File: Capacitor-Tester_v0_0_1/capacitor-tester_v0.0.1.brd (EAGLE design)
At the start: 67 x 45 mm, 34 parts, among them IC1 AD8531ARZ, IC2 MC34063EBD-TR, IC3 DAC6571IDBVT, IC5 AD8397ARDZ, J1 USB4125-GF-A-0190_REVA2, J2 DS1044-140G, J4 250-103, U1 AD5933, Y1 LFSPXO018034

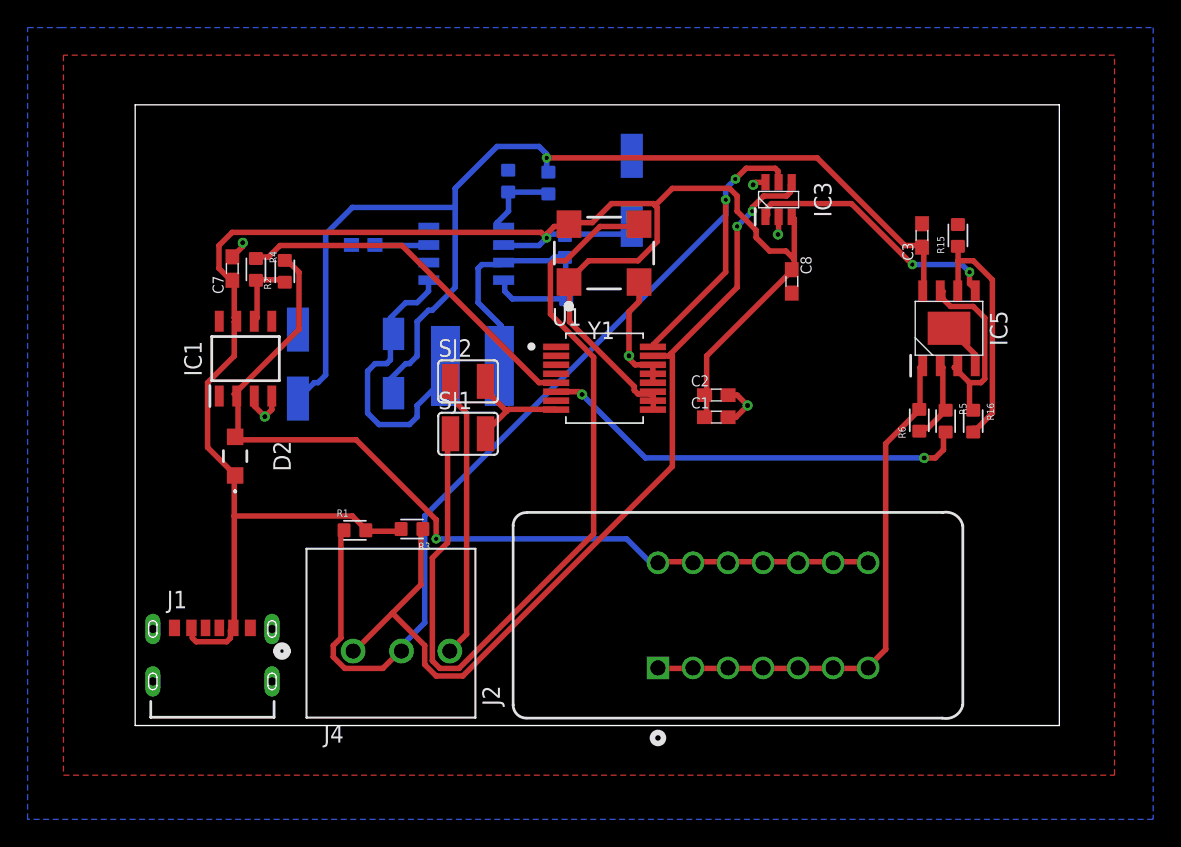
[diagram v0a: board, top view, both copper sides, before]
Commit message: v0.0.1 - CMD renumber + tnames + bnames
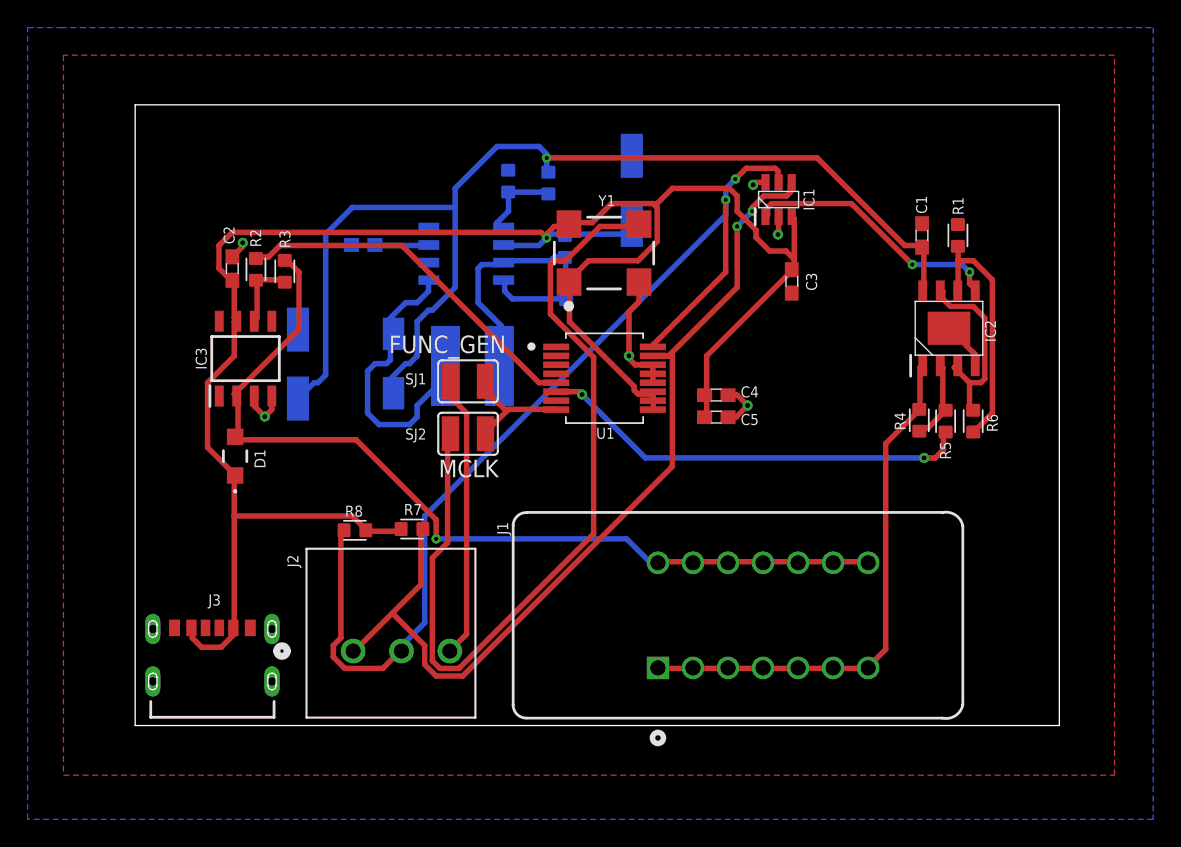
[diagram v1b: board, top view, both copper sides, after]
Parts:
- removed IC5: AD8397ARDZ, AD8397ARDZ:SOIC127P600X175-9N
- removed J4: 250-103, custom_library:CONN3_250-103_WAG
- removed R15, R16: 10k-1%, custom_library:R0603
- added IC4: MC34063EBD-TR, MC34063EBD-TR:SOIC127P600X175-8N
- added J3: USB4125-GF-A-0190_REVA2, USB-C-6Pin:GCT_USB4125-GF-A-0190_REVA2
- added R7, R8: DNP-4k7-1%, custom_library:R0603
- C2: value 10u -> 100n
- C3: value 100n -> 10u
- C4: value 270u / 16V -> 10u; device EEEFKC271XSP:EEE0JA331XP -> custom_library:C0603
- C5: value 270u / 16V -> 100n; device EEEFKC271XSP:EEE0JA331XP -> custom_library:C0603
- C6: value 560p -> 270u / 16V; device custom_library:C0603 -> EEEFKC271XSP:EEE0JA331XP
- C7: value 100n -> 560p
- C8: value 10u -> 270u / 16V; device custom_library:C0603 -> EEEFKC271XSP:EEE0JA331XP
- D1: value SS14 -> PMEG6020ER,115; device SS14:DIOM5227X270N -> PMEG6020ER_115:PMEG6020ER115
- D2: value PMEG6020ER,115 -> SS14; device PMEG6020ER_115:PMEG6020ER115 -> SS14:DIOM5227X270N
- IC1: value AD8531ARZ -> DAC6571IDBVT; device AD8531ARZ:SOIC127P600X175-8N -> DAC6571IDBVT:SOT95P280X145-6N
- IC2: value MC34063EBD-TR -> AD8397ARDZ; device MC34063EBD-TR:SOIC127P600X175-8N -> AD8397ARDZ:SOIC127P600X175-9N
- IC3: value DAC6571IDBVT -> AD8531ARZ; device DAC6571IDBVT:SOT95P280X145-6N -> AD8531ARZ:SOIC127P600X175-8N
- J1: value USB4125-GF-A-0190_REVA2 -> DS1044-140G; device USB-C-6Pin:GCT_USB4125-GF-A-0190_REVA2 -> DS1044-140G:CONNFLY_DS1044-140G
- J2: value DS1044-140G -> 250-103; device DS1044-140G:CONNFLY_DS1044-140G -> custom_library:CONN3_250-103_WAG
- R1, R3: value DNP-4k7-1% -> 10k-1%
- R10: value 1k-1% -> R133-1%
- R11: value R133-1% -> 8k66-1%
- R12: value 180R-1% -> 1k-1%
- R2: value 10k-1% -> DNP-10k-1%
- R4: value DNP-10k-1% -> 1k-1%
- R6: value 1k-1% -> 10k-1%
- R9: value 8k66-1% -> 180R-1%
- moved R4 49.3 mm to (56.8, 22.1), turned to 90 degrees
- moved R1 48.7 mm to (59.6, 35.5), turned to 90 degrees
- moved IC1 40.3 mm to (46.6, 38.1)
- moved IC3 40.3 mm to (8.00, 26.6)
- moved J1 40.1 mm to (45.5, 7.99), turned to 90 degrees
- moved C2 36.3 mm to (7.05, 33.1), turned to 90 degrees
- moved IC2 35.4 mm to (59.0, 28.8), flipped to the top, turned to 90 degrees
- moved C4 30.4 mm to (42.1, 24.0), flipped to the top, turned to 0 degrees
- moved J2 29.8 mm to (15.8, 5.40), turned to 0 degrees
- moved R3 20.8 mm to (10.8, 32.9), turned to 90 degrees
- moved C1 19.9 mm to (57.0, 35.5), turned to 90 degrees
- moved C5 17.6 mm to (42.1, 22.4), flipped to the top, turned to 0 degrees
- moved C8 13.3 mm to (36.0, 38.8), flipped to the bottom, turned to 90 degrees
- moved D1 13.3 mm to (7.25, 19.5), flipped to the top
- moved D2 13.3 mm to (18.7, 26.2), flipped to the bottom
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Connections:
- net +12V: now also C1.1, C6.1, D2.1, IC2.8, R11.1; no longer C3.1, C4.1, D1.1, IC5.8, R9.1
- net +5V: now also C3.1, C4.1, D1.1, IC1.3, IC3.7, IC4.6, J3.A9, J3.B9, R10.1, R7.2, R8.2; no longer C1.1, C7.1, D2.1, IC1.7, IC2.6, IC3.3, J1.A9, J1.B9, R1.2, R11.1, R3.2
- net DAC_OUT: now also IC1.1, IC2.5; no longer IC3.1, IC5.5
- net FUNC_GEN: now also J2.3, SJ1.1; no longer J4.3, SJ2.1
- net GND: now also IC1.2, IC1.6, IC2.9, IC3.3, IC3.4, IC4.2, IC4.4, J3.A12, J3.B12, J3.S1, J3.S2, J3.S3, J3.S4, R1.2, R12.2; no longer IC1.3, IC1.4, IC2.2, IC3.2, IC3.6, IC5.4, IC5.9, J1.A12, J1.B12, J1.S1, J1.S2, J1.S3, J1.S4, R10.2, R15.2
- net MCLK: now also SJ2.1; no longer SJ1.1
- net N$1: now also IC3.6, R2.2, R3.1; no longer IC1.6, R2.1, R4.2
- net N$10: now also C7.1, IC4.3; no longer C6.1, IC2.3
- net N$11: now also IC4.7, R10.2, R9.2; no longer IC2.7, R11.2, R12.2
- net N$13: now also IC2.6, R1.1, R6.2; no longer IC5.6, R15.1, R16.2
- net N$4: now also IC2.2, R4.1; no longer IC5.2, R6.1
- net N$5: now also D2.2, IC4.1; no longer D1.2, IC2.1
- net N$7: now also IC4.5, R11.2, R12.1; no longer IC2.5, R10.1, R9.2
- net N$8: now also IC4.8, R9.1; no longer IC2.8, R12.1
- net SCL: now also IC1.5, J2.2, R8.1; no longer IC3.5, J4.2, R1.1
- net SDA: now also IC1.4, J2.1, R7.1; no longer IC3.4, J4.1, R3.1
- net UZA_OUT: now also IC2.1, J1.1, J1.2, J1.3, J1.4, J1.5, J1.6, J1.7, R4.2; no longer IC5.1, J2.1, J2.2, J2.3, J2.4, J2.5, J2.6, J2.7, R6.2
- net UZB_OUT: now also IC2.3, IC2.7, R6.1; no longer IC5.3, IC5.7, R16.1
- net VIN: now also R2.1; no longer R4.1
- net Z_OUT: now also D1.2, IC3.2, J1.10, J1.11, J1.12, J1.13, J1.14, J1.8, J1.9, R3.2; no longer D2.2, IC1.2, J2.10, J2.11, J2.12, J2.13, J2.14, J2.8, J2.9, R2.2
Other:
- board text added: "FUNC_GEN"
- board text added: "MCLK"

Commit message: v0.0.1 - Revert to commit b06d3d6
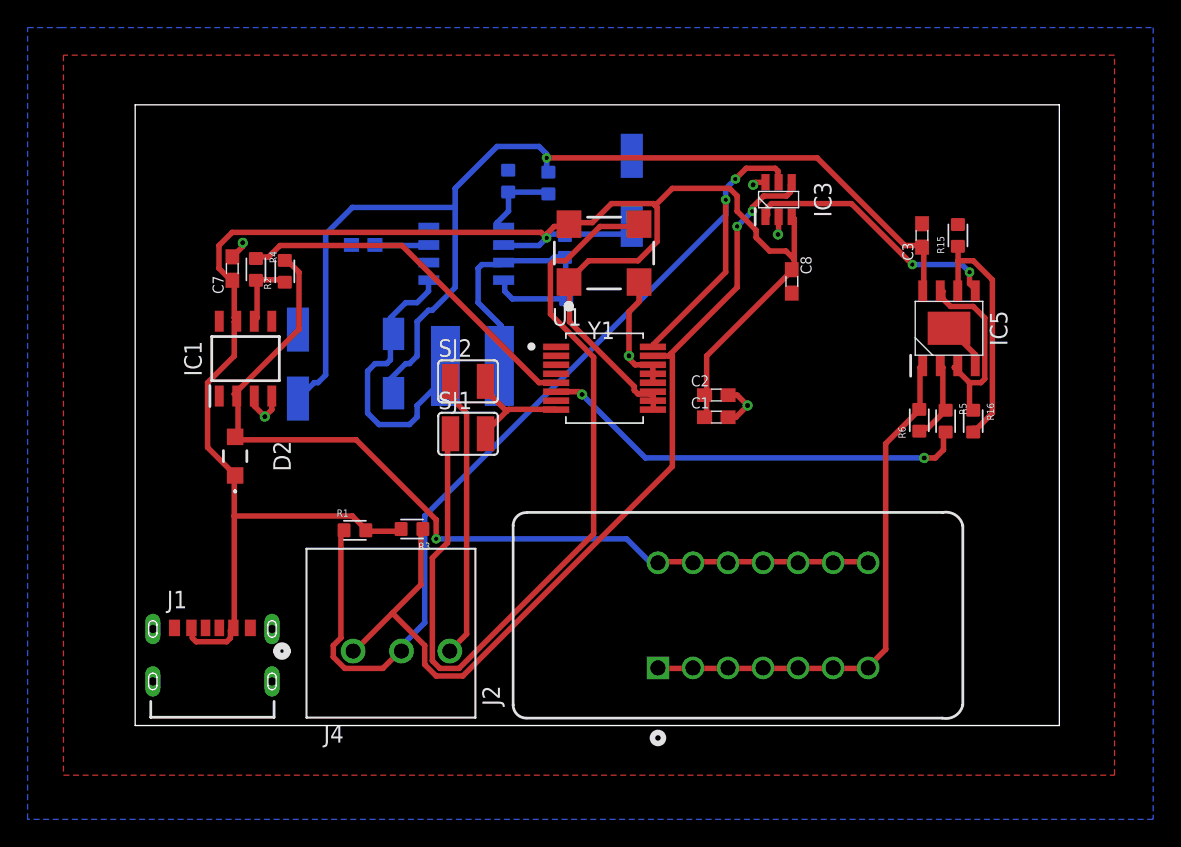
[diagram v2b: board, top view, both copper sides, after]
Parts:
- removed IC4: MC34063EBD-TR, MC34063EBD-TR:SOIC127P600X175-8N
- removed J3: USB4125-GF-A-0190_REVA2, USB-C-6Pin:GCT_USB4125-GF-A-0190_REVA2
- removed R7, R8: DNP-4k7-1%, custom_library:R0603
- added IC5: AD8397ARDZ, AD8397ARDZ:SOIC127P600X175-9N
- added J4: 250-103, custom_library:CONN3_250-103_WAG
- added R15, R16: 10k-1%, custom_library:R0603
- C2: value 100n -> 10u
- C3: value 10u -> 100n
- C4: value 10u -> 270u / 16V; device custom_library:C0603 -> EEEFKC271XSP:EEE0JA331XP
- C5: value 100n -> 270u / 16V; device custom_library:C0603 -> EEEFKC271XSP:EEE0JA331XP
- C6: value 270u / 16V -> 560p; device EEEFKC271XSP:EEE0JA331XP -> custom_library:C0603
- C7: value 560p -> 100n
- C8: value 270u / 16V -> 10u; device EEEFKC271XSP:EEE0JA331XP -> custom_library:C0603
- D1: value PMEG6020ER,115 -> SS14; device PMEG6020ER_115:PMEG6020ER115 -> SS14:DIOM5227X270N
- D2: value SS14 -> PMEG6020ER,115; device SS14:DIOM5227X270N -> PMEG6020ER_115:PMEG6020ER115
- IC1: value DAC6571IDBVT -> AD8531ARZ; device DAC6571IDBVT:SOT95P280X145-6N -> AD8531ARZ:SOIC127P600X175-8N
- IC2: value AD8397ARDZ -> MC34063EBD-TR; device AD8397ARDZ:SOIC127P600X175-9N -> MC34063EBD-TR:SOIC127P600X175-8N
- IC3: value AD8531ARZ -> DAC6571IDBVT; device AD8531ARZ:SOIC127P600X175-8N -> DAC6571IDBVT:SOT95P280X145-6N
- J1: value DS1044-140G -> USB4125-GF-A-0190_REVA2; device DS1044-140G:CONNFLY_DS1044-140G -> USB-C-6Pin:GCT_USB4125-GF-A-0190_REVA2
- J2: value 250-103 -> DS1044-140G; device custom_library:CONN3_250-103_WAG -> DS1044-140G:CONNFLY_DS1044-140G
- R1, R3: value 10k-1% -> DNP-4k7-1%
- R10: value R133-1% -> 1k-1%
- R11: value 8k66-1% -> R133-1%
- R12: value 1k-1% -> 180R-1%
- R2: value DNP-10k-1% -> 10k-1%
- R4: value 1k-1% -> DNP-10k-1%
- R6: value 10k-1% -> 1k-1%
- R9: value 180R-1% -> 8k66-1%
- moved R4 49.3 mm to (8.75, 33.1), turned to 270 degrees
- moved R1 48.7 mm to (15.9, 14.2), turned to 0 degrees
- moved IC1 40.3 mm to (8.00, 26.6)
- moved IC3 40.3 mm to (46.6, 38.1)
- moved J1 40.1 mm to (5.60, 4.00), turned to 0 degrees
- moved C2 36.3 mm to (42.1, 24.0), turned to 0 degrees
- moved IC2 35.4 mm to (24.0, 34.2), flipped to the bottom, turned to 180 degrees
- moved C4 30.4 mm to (11.8, 26.2), flipped to the bottom, turned to 90 degrees
- moved J2 29.8 mm to (45.5, 7.99), turned to 90 degrees
- moved R3 20.8 mm to (20.1, 14.2), turned to 180 degrees
- moved C1 19.9 mm to (42.1, 22.4), turned to 0 degrees
- moved C5 17.6 mm to (36.0, 38.8), flipped to the bottom, turned to 90 degrees
- moved C8 13.3 mm to (47.6, 32.2), flipped to the top, turned to 270 degrees
- moved D1 13.3 mm to (18.7, 26.2), flipped to the bottom
- moved D2 13.3 mm to (7.25, 19.5), flipped to the top
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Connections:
- net +12V: now also C3.1, C4.1, D1.1, IC5.8, R9.1; no longer C1.1, C6.1, D2.1, IC2.8, R11.1
- net +5V: now also C1.1, C7.1, D2.1, IC1.7, IC2.6, IC3.3, J1.A9, J1.B9, R1.2, R11.1, R3.2; no longer C3.1, C4.1, D1.1, IC1.3, IC3.7, IC4.6, J3.A9, J3.B9, R10.1, R7.2, R8.2
- net DAC_OUT: now also IC3.1, IC5.5; no longer IC1.1, IC2.5
- net FUNC_GEN: now also J4.3, SJ2.1; no longer J2.3, SJ1.1
- net GND: now also IC1.3, IC1.4, IC2.2, IC3.2, IC3.6, IC5.4, IC5.9, J1.A12, J1.B12, J1.S1, J1.S2, J1.S3, J1.S4, R10.2, R15.2; no longer IC1.2, IC1.6, IC2.9, IC3.3, IC3.4, IC4.2, IC4.4, J3.A12, J3.B12, J3.S1, J3.S2, J3.S3, J3.S4, R1.2, R12.2
- net MCLK: now also SJ1.1; no longer SJ2.1
- net N$1: now also IC1.6, R2.1, R4.2; no longer IC3.6, R2.2, R3.1
- net N$10: now also C6.1, IC2.3; no longer C7.1, IC4.3
- net N$11: now also IC2.7, R11.2, R12.2; no longer IC4.7, R10.2, R9.2
- net N$13: now also IC5.6, R15.1, R16.2; no longer IC2.6, R1.1, R6.2
- net N$4: now also IC5.2, R6.1; no longer IC2.2, R4.1
- net N$5: now also D1.2, IC2.1; no longer D2.2, IC4.1
- net N$7: now also IC2.5, R10.1, R9.2; no longer IC4.5, R11.2, R12.1
- net N$8: now also IC2.8, R12.1; no longer IC4.8, R9.1
- net SCL: now also IC3.5, J4.2, R1.1; no longer IC1.5, J2.2, R8.1
- net SDA: now also IC3.4, J4.1, R3.1; no longer IC1.4, J2.1, R7.1
- net UZA_OUT: now also IC5.1, J2.1, J2.2, J2.3, J2.4, J2.5, J2.6, J2.7, R6.2; no longer IC2.1, J1.1, J1.2, J1.3, J1.4, J1.5, J1.6, J1.7, R4.2
- net UZB_OUT: now also IC5.3, IC5.7, R16.1; no longer IC2.3, IC2.7, R6.1
- net VIN: now also R4.1; no longer R2.1
- net Z_OUT: now also D2.2, IC1.2, J2.10, J2.11, J2.12, J2.13, J2.14, J2.8, J2.9, R2.2; no longer D1.2, IC3.2, J1.10, J1.11, J1.12, J1.13, J1.14, J1.8, J1.9, R3.2
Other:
- board text removed: "FUNC_GEN"
- board text removed: "MCLK"
